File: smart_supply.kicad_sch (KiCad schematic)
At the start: 0 parts

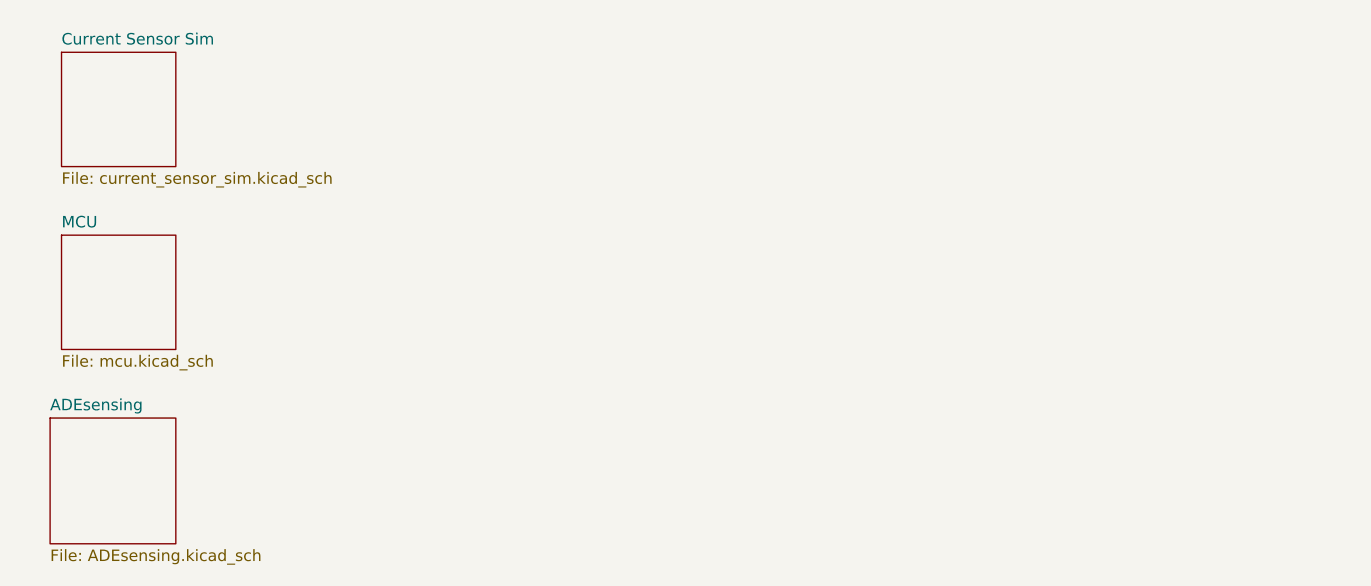
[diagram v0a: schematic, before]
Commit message: ade7953 breakout board
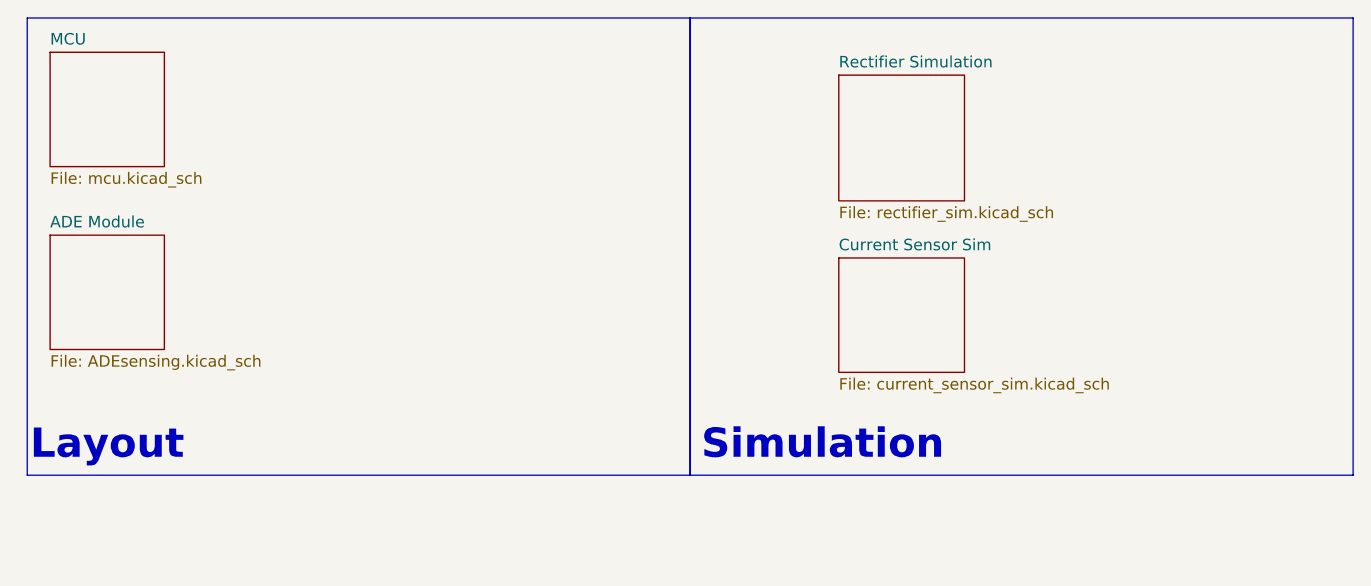
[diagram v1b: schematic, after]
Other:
- sheet ADEsensing renamed ADE Module
- added sheet Rectifier Simulation (rectifier_sim.kicad_sch)
- note added: "Layout"
- note added: "Simulation"
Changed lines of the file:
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@@
 	(generator_version "10.0")
 	(paper "A4")
-	(sheet
-		(at 21.59 62.23)
-		(size 13.97 13.97)
-		(exclude_from_sim no)
-		(in_bom yes)
-		(on_board yes)
-		(dnp no)
-		(fields_autoplaced yes)
-		(stroke
-			(width 0.1524)
-			(type solid)
-		)
-		(fill
-			(color 0 0 0 0)
-		)
-		(property "Sheetname" "ADEsensing"
-			(at 21.59 61.5184 0)
-			(show_name no)
-			(do_not_autoplace no)
-			(effects
-				(font
-					(size 1.27 1.27)
-				)
-				(justify left bottom)
-			)
-		)
-		(property "Sheetfile" "ADEsensing.kicad_sch"
-			(at 21.59 76.7846 0)
-			(show_name no)
-			(do_not_autoplace no)
-			(effects
-				(font
-					(size 1.27 1.27)
-				)
-				(justify left top)
-			)
-		)
-		(instances
-			(project "smart_supply"
-				(path "/487ef637-7a03-4925-80c1-798e0c6f0bbd"
-					(page "4")
-				)
-			)
-		)
-	)
-	(sheet
-		(at 22.86 21.59)
-		(size 12.7 12.7)
-		(exclude_from_sim no)
-		(in_bom no)
-		(on_board no)
-		(dnp no)
-		(fields_autoplaced yes)
-		(stroke
-			(width 0.1524)
-			(type solid)
-		)
-		(fill
-			(color 0 0 0 0)
-		)
-		(property "Sheetname" "Current Sensor Sim"
-			(at 22.86 20.8784 0)
-			(show_name no)
-			(do_not_autoplace no)
-			(effects
-				(font
-					(size 1.27 1.27)
-				)
-				(justify left bottom)
-			)
-		)
-		(property "Sheetfile" "current_sensor_sim.kicad_sch"
-			(at 22.86 34.8746 0)
-			(show_name no)
-			(do_not_autoplace no)
-			(effects
-				(font
-					(size 1.27 1.27)
-				)
-				(justify left top)
-			)
-		)
-		(instances
-			(project "smart_supply"
-				(path "/487ef637-7a03-4925-80c1-798e0c6f0bbd"
-					(page "2")
-				)
-			)
-		)
-	)
-	(sheet
-		(at 22.86 41.91)
+	(rectangle
+		(start 92.71 17.78)
+		(end 166.37 68.58)
+		(stroke
+			(width 0)
+			(type default)
+		)
+		(fill
+			(type none)
+		)
+	)
+	(rectangle
+		(start 19.05 17.78)
+		(end 92.71 68.58)
+		(stroke
+			(width 0)
+			(type default)
+		)
+		(fill
+			(type none)
+		)
+	)
+	(text "Simulation"
+		(exclude_from_sim no)
+		(at 107.442 65.278 0)
+		(effects
+			(font
+				(size 3.2512 3.2512)
+				(thickness 0.6502)
+				(bold yes)
+				(color 255 153 0 1)
+			)
+		)
+	)
+	(text "Layout"
+		(exclude_from_sim no)
+		(at 27.94 65.278 0)
+		(effects
+			(font
+				(size 3.2512 3.2512)
+				(thickness 0.6502)
+				(bold yes)
+				(color 0 0 255 1)
+			)
+		)
+	)
+	(sheet
+		(at 21.59 41.91)
 		(size 12.7 12.7)
 		(exclude_from_sim yes)
@@
 			(color 0 0 0 0)
 		)
+		(property "Sheetname" "ADE Module"
+			(at 21.59 41.1984 0)
+			(show_name no)
+			(do_not_autoplace no)
+			(effects
+				(font
+					(size 1.27 1.27)
+				)
+				(justify left bottom)
+			)
+		)
+		(property "Sheetfile" "ADEsensing.kicad_sch"
+			(at 21.59 55.1946 0)
+			(show_name no)
+			(do_not_autoplace no)
+			(effects
+				(font
+					(size 1.27 1.27)
+				)
+				(justify left top)
+			)
+		)
+		(instances
+			(project "smart_supply"
+				(path "/487ef637-7a03-4925-80c1-798e0c6f0bbd"
+					(page "5")
+				)
+			)
+		)
+	)
+	(sheet
+		(at 109.22 44.45)
+		(size 13.97 12.7)
+		(exclude_from_sim no)
+		(in_bom no)
+		(on_board no)
+		(dnp no)
+		(fields_autoplaced yes)
+		(stroke
+			(width 0.1524)
+			(type solid)
+		)
+		(fill
+			(color 0 0 0 0)
+		)
+		(property "Sheetname" "Current Sensor Sim"
+			(at 109.22 43.7384 0)
+			(show_name no)
+			(do_not_autoplace no)
+			(effects
+				(font
+					(size 1.27 1.27)
+				)
+				(justify left bottom)
+			)
+		)
+		(property "Sheetfile" "current_sensor_sim.kicad_sch"
+			(at 109.22 57.7346 0)
+			(show_name no)
+			(do_not_autoplace no)
+			(effects
+				(font
+					(size 1.27 1.27)
+				)
+				(justify left top)
+			)
+		)
+		(instances
+			(project "smart_supply"
+				(path "/487ef637-7a03-4925-80c1-798e0c6f0bbd"
+					(page "2")
+				)
+			)
+		)
+	)
+	(sheet
+		(at 109.22 24.13)
+		(size 13.97 13.97)
+		(exclude_from_sim no)
+		(in_bom no)
+		(on_board no)
+		(dnp no)
+		(fields_autoplaced yes)
+		(stroke
+			(width 0.1524)
+			(type solid)
+		)
+		(fill
+			(color 0 0 0 0)
+		)
+		(property "Sheetname" "Rectifier Simulation"
+			(at 109.22 23.4184 0)
+			(show_name no)
+			(do_not_autoplace no)
+			(effects
+				(font
+					(size 1.27 1.27)
+				)
+				(justify left bottom)
+			)
+		)
+		(property "Sheetfile" "rectifier_sim.kicad_sch"
+			(at 109.22 38.6846 0)
+			(show_name no)
+			(do_not_autoplace no)
+			(effects
+				(font
+					(size 1.27 1.27)
+				)
+				(justify left top)
+			)
+		)
+		(instances
+			(project "smart_supply"
+				(path "/487ef637-7a03-4925-80c1-798e0c6f0bbd"
+					(page "3")
+				)
+			)
+		)
+	)
+	(sheet
+		(at 21.59 21.59)
+		(size 12.7 12.7)
+		(exclude_from_sim yes)
+		(in_bom no)
+		(on_board no)
+		(dnp no)
+		(fields_autoplaced yes)
+		(stroke
+			(width 0.1524)
+			(type solid)
+		)
+		(fill
+			(color 0 0 0 0)
+		)
 		(property "Sheetname" "MCU"
-			(at 22.86 41.1984 0)
+			(at 21.59 20.8784 0)
 			(show_name no)
 			(do_not_autoplace no)
@@
 		)
 		(property "Sheetfile" "mcu.kicad_sch"
-			(at 22.86 55.1946 0)
-			(show_name no)
-			(do_not_autoplace no)
-			(effects
-				(font
-					(size 1.27 1.27)
-				)
-				(justify left top)
-			)
-		)
-		(instances
-			(project "smart_supply"
-				(path "/487ef637-7a03-4925-80c1-798e0c6f0bbd"
-					(page "3")
-				)
-			)
+			(at 21.59 34.8746 0)
+			(show_name no)
+			(do_not_autoplace no)
+			(effects
+				(font
+					(size 1.27 1.27)
+				)
+				(justify left top)
+			)
+		)
+		(instances
+			(project "smart_supply"
+				(path "/487ef637-7a03-4925-80c1-798e0c6f0bbd"
+					(page "4")
+				)
+			)
